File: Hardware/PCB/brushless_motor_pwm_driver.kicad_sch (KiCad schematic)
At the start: 3 parts, among them U5 74LVC2T45DC

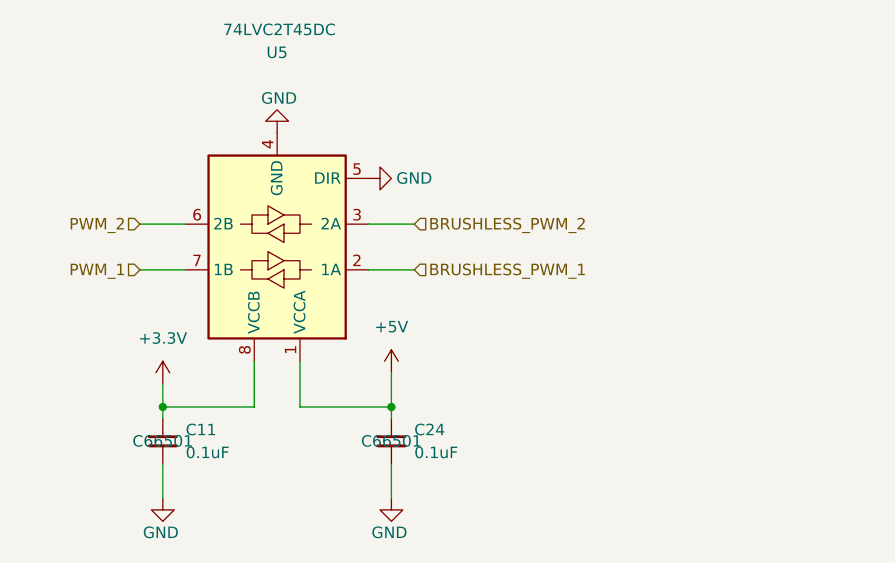
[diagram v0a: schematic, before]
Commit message: done with this, placed order
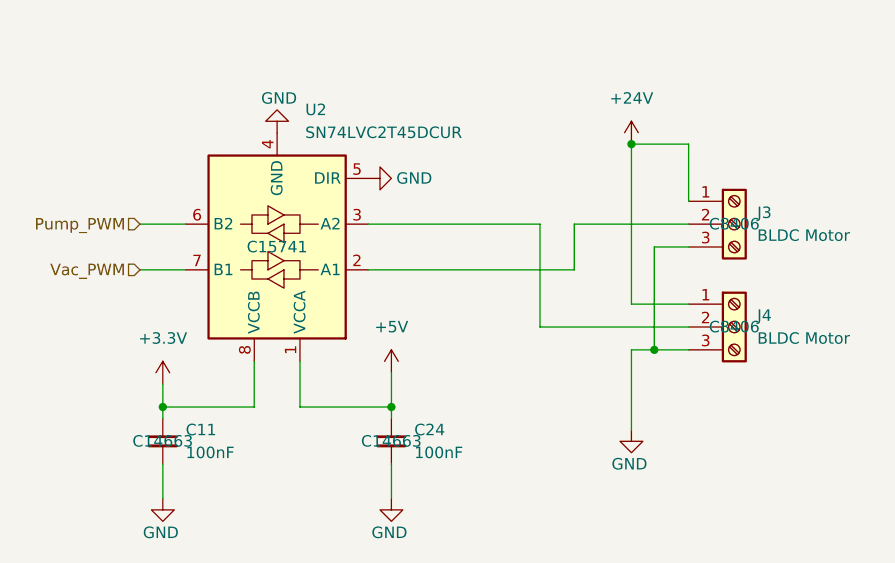
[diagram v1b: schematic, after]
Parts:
- removed U5: 74LVC2T45DC, Package_SO:VSSOP-8_2.3x2mm_P0.5mm, symbol Logic_LevelTranslator:74LVCH2T45DC
- added J3, J4: BLDC Motor, Vendor_Footprints:CONN_WJ15EDGRC-3.81-3P, symbol Connector:Screw_Terminal_01x03
- added U2: SN74LVC2T45DCUR, Package_SO:VSSOP-8_2.3x2mm_P0.5mm, symbol Logic_LevelTranslator:SN74LVC2T45DCUR
- C11, C24: value 0.1uF -> 100nF; LCSC C66501 -> C14663; MPN CL10B104KO8NNNC -> CC0603KRX7R9BB104; Manufacturer Samsung Electro-Mechanics -> YAGEO
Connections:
- net +3.3V: now also U2.8 (VCCB)
- net +5V: now also U2.1 (VCCA)
- net GND: now also J3.3 (Pin_3), J4.3 (Pin_3), U2.4 (GND), U2.5 (DIR)
- new net: J3.2 (Pin_2), U2.2 (A1)
- new net: J4.2 (Pin_2), U2.3 (A2)
- new net +24V: J3.1 (Pin_1), J4.1 (Pin_1)
- new net Pump_PWM: U2.6 (B2)
- new net Vac_PWM: U2.7 (B1)
